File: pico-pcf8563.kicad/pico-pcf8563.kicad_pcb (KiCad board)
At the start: 2 copper layers, 21 x 18.6 mm, 13 parts, among them J1 Stemma-QT_Qwicc, J2 Ext_Conn, J4 Pico Pin 1-7, J5 Pico Pin 40-34, U1 PCF8563T, Y1 Crystal

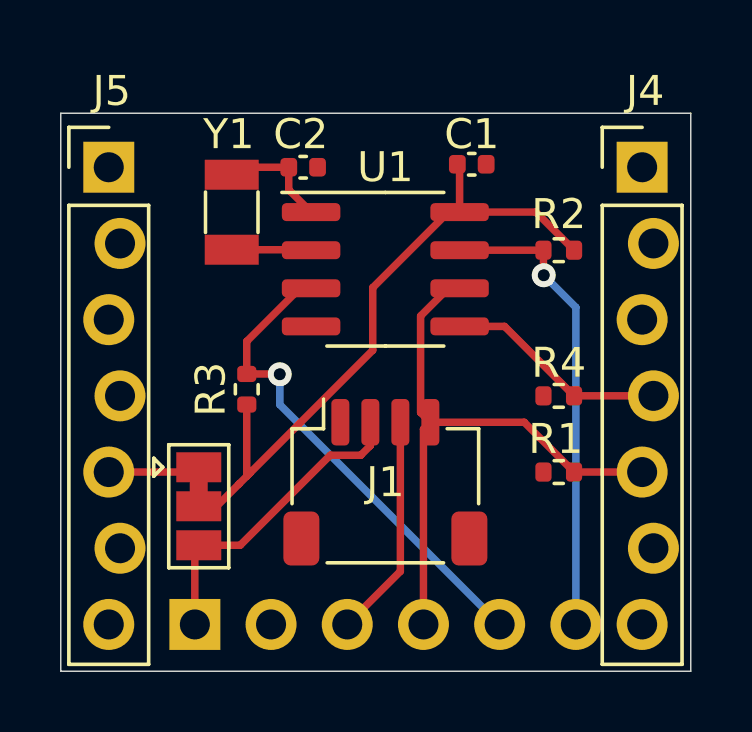
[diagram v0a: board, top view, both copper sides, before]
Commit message: Rev2
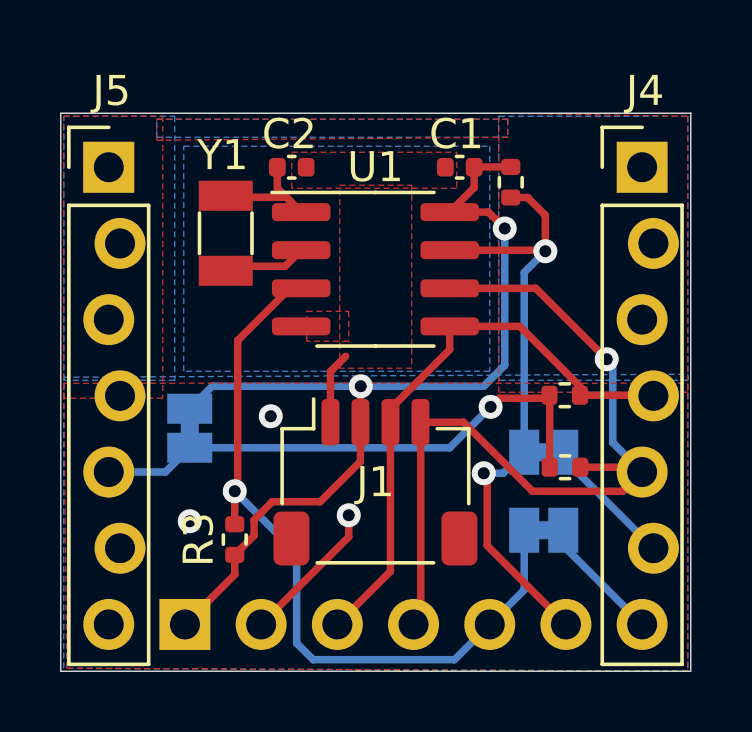
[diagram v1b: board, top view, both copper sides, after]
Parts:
- added JP2: ~{INT}_Jumper, Jumper:SolderJumper-2_P1.3mm_Bridged_Pad1.0x1.5mm, B.Cu at (114.5, 109.5)
- added JP3: COUT_Jumper, Jumper:SolderJumper-2_P1.3mm_Bridged_Pad1.0x1.5mm, B.Cu at (114.5, 112.1)
- JP1: value VDD_SEL -> 3V3_Jumper; footprint Jumper:SolderJumper-3_P1.3mm_Bridged12_Pad1.0x1.5mm -> Jumper:SolderJumper-2_P1.3mm_Bridged_Pad1.0x1.5mm; moved to B.Cu
- moved R3 5.03 mm to (104.2, 112.4)
- moved R2 2.77 mm to (113.4, 100.5), turned to 90 degrees
- moved JP1 2.62 mm to (102.7, 108.7), turned to 90 degrees
- moved Y1 0.73 mm to (103.9, 102.2)
- moved C1 0.41 mm to (111.7, 100.0), turned to 180 degrees
- moved C2 0.38 mm to (106.1, 100.0)
- moved J1 0.33 mm to (108.9, 110.5)
- moved J2 0.33 mm to (102.5, 115.2)
- moved U1 0.33 mm to (108.9, 103.4)
- moved R1 0.26 mm to (115.2, 110.0)
- moved R4 0.20 mm to (115.2, 107.6)
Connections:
- C1 pad 1: VDD -> VCC
- J4 pad 6: unconnected-(J4-Pad6) -> /GP4
- J4 pad 7: unconnected-(J4-Pad7) -> /GP5
- JP1 pad 2: VDD -> VCC
- R2 pad 2: VDD -> VCC
- R3 pad 2: VDD -> VCC
- U1 pad 8: VDD -> VCC
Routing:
- net VDD: track 22.3 -> 0.00 mm
- net VCC: track 10.6 -> 32.1 mm, vias 0 -> 2
- net +3V3: track 3.07 -> 18.2 mm, vias 0 -> 1
- net /~{INT}: track 16.4 -> 25.7 mm
- net /SCL: track 19.9 -> 28.0 mm, vias 0 -> 1
- net GND: track 0.00 -> 7.26 mm, vias 0 -> 3
- net /COUT: track 15.7 -> 20.6 mm, vias 1 -> 2
- net /SDA: track 14.9 -> 19.4 mm
- net /GP4: track 0.00 -> 4.45 mm
- net /GP5: track 0.00 -> 4.23 mm
- added copper zone on B.Cu, net GND
- added copper zone on F.Cu, net GND
